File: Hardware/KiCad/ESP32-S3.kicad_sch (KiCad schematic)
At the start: 33 parts, among them J1 UJ20-C-H-G-SMT-1-P16-TR, J4 RJ45, J5 Conn_TagConnect_TC2030-NL_ESP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, U1 ESP32-S3-WROOM-1, U5 WE-TVS-82400102, U7 AP7333-33SRG-7

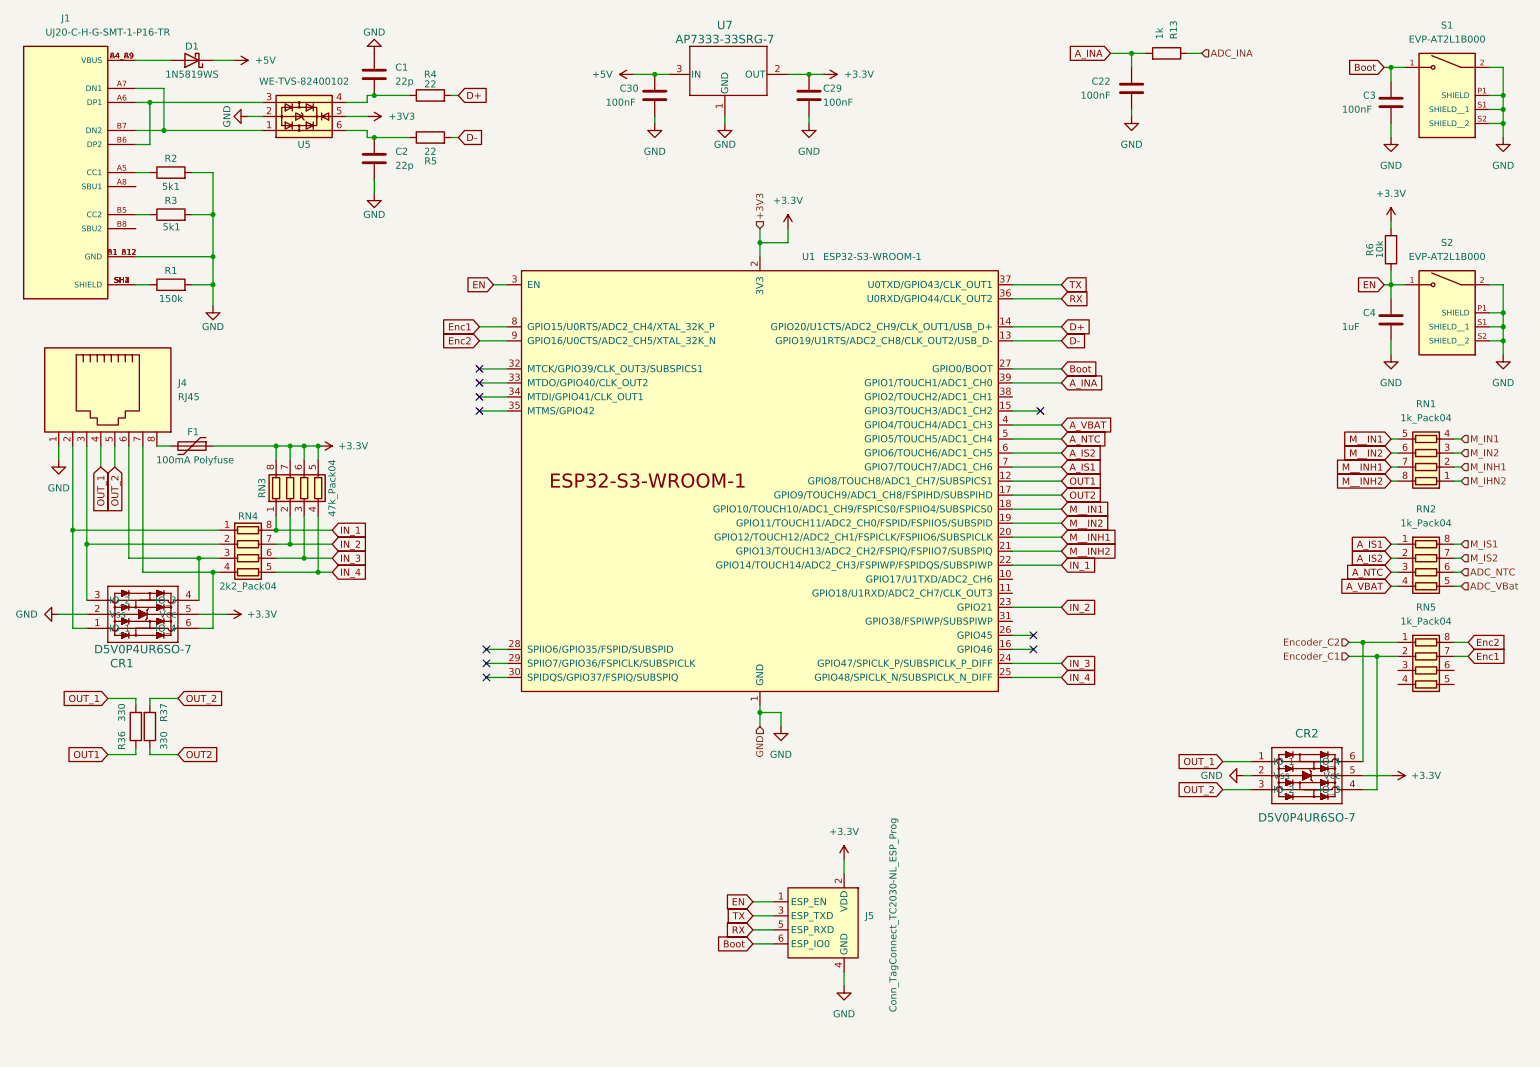
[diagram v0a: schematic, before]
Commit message: begin routing
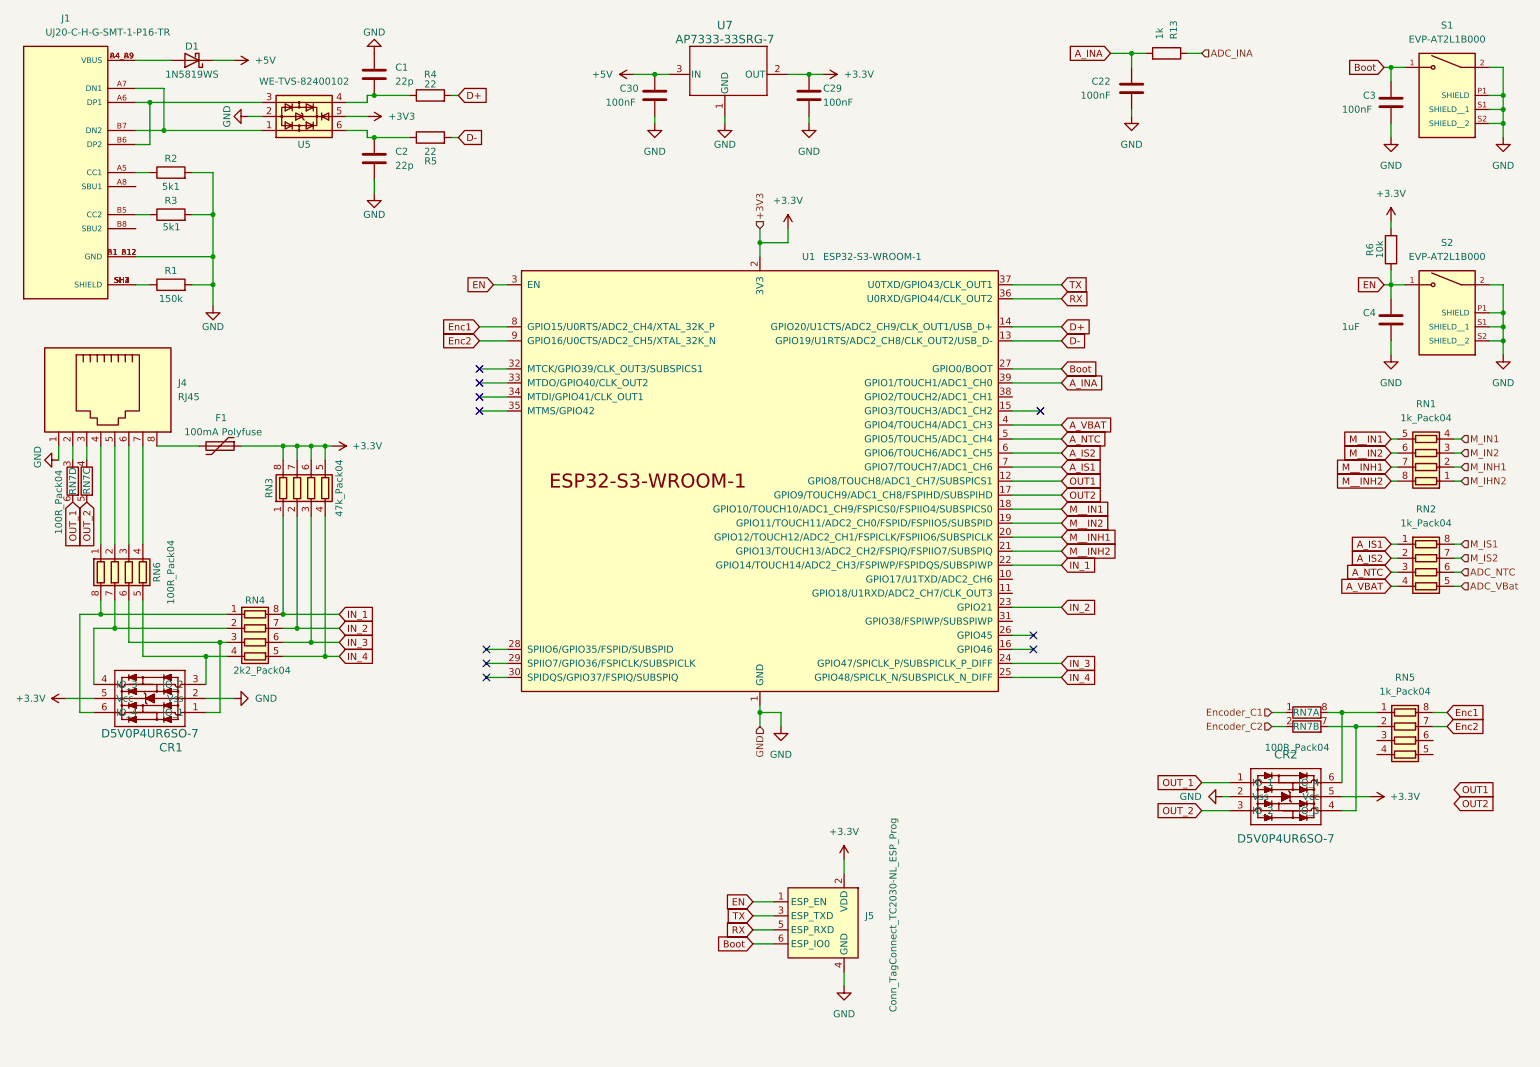
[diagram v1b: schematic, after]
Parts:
- removed R36, R37: 330, Resistor_SMD:R_0603_1608Metric, symbol Device:R
- added RN6: 100R_Pack04, BugWiper_lib:BO_CAY16, symbol Device:R_Pack04
- added RN7: 100R_Pack04, Resistor_THT:R_Array_SIP8, symbol Device:R_Pack04_Split
- D1: footprint Diode_SMD:D_SOD-323 -> Diode_SMD:D_SOD-323_HandSoldering
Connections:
- net Enc1: now also RN5.8 (R1.2); no longer RN5.7 (R2.2)
- net Enc2: now also RN5.7 (R2.2); no longer RN5.8 (R1.2)
- net Encoder_C1: now also RN7.1 (R1.1); no longer CR2.4 (IO_3), RN5.2 (R2.1)
- net Encoder_C2: now also RN7.2 (R2.1); no longer CR2.6 (IO_4), RN5.1 (R1.1)
- net OUT_1: now also RN7.6 (R3.2); no longer J4.4
- net OUT_2: now also RN7.5 (R4.2); no longer J4.5
- new net: CR1.6 (IO_4), RN4.1 (R1.1), RN6.8 (R1.2)
- new net: CR1.4 (IO_3), RN4.2 (R2.1), RN6.7 (R2.2)
- new net: CR1.1 (IO_1), RN4.3 (R3.1), RN6.6 (R3.2)
- new net: CR1.3 (IO_2), RN4.4 (R4.1), RN6.5 (R4.2)
- new net: J4.2, RN7.3 (R3.1)
- new net: J4.4, RN6.1 (R1.1)
- new net: J4.5, RN6.2 (R2.1)
- new net: J4.6, RN6.3 (R3.1)
- new net: J4.7, RN6.4 (R4.1)
- new net: CR2.4 (IO_3), RN5.2 (R2.1), RN7.7 (R2.2)
- new net: J4.3, RN7.4 (R4.1)
- new net: CR2.6 (IO_4), RN5.1 (R1.1), RN7.8 (R1.2)
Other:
- moved on the sheet: CR1, CR2, F1, RN3, RN4, RN5
